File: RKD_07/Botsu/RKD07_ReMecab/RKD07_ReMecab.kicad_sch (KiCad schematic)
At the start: 16 parts, among them J2 Conn_01x24, J3 Qwiic_RA, J4 Conn_01x06, J5 Conn_01x02_Socket, J7 Conn_01x08, J8 Conn_01x06, SW41 SW_Push, U1 Pico

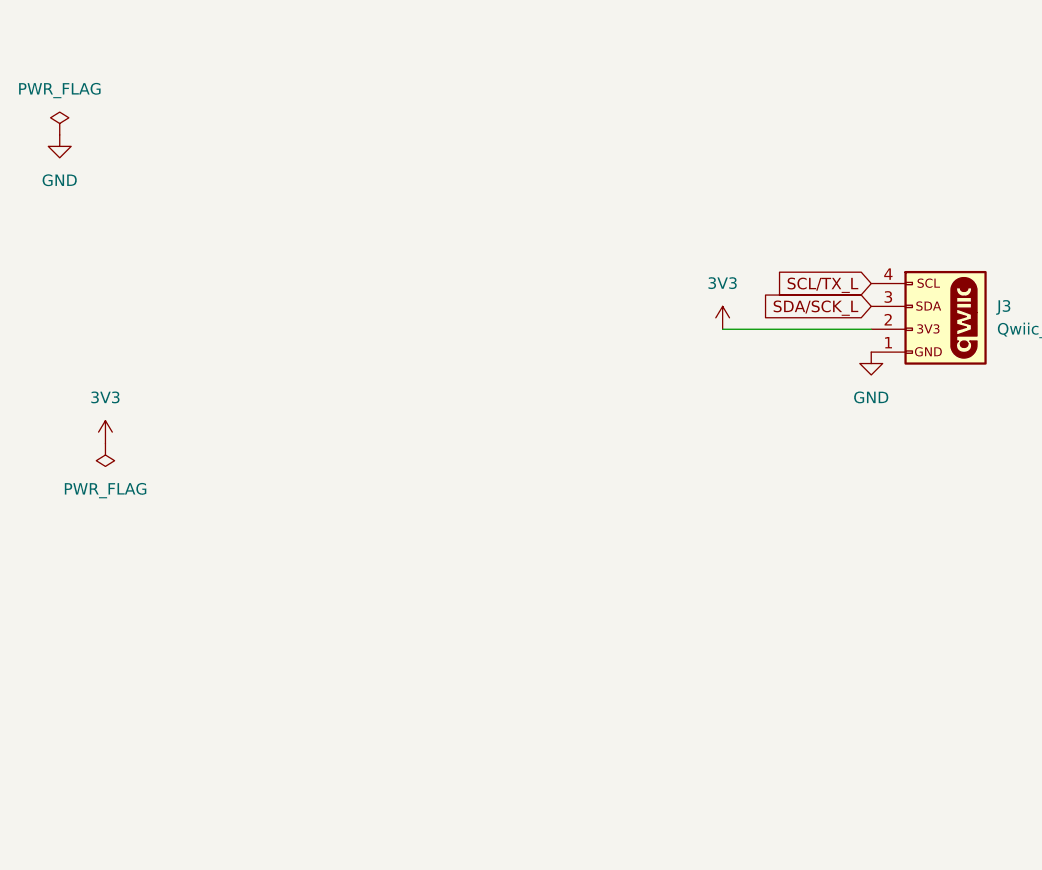
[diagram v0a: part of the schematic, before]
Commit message: Update Remecab
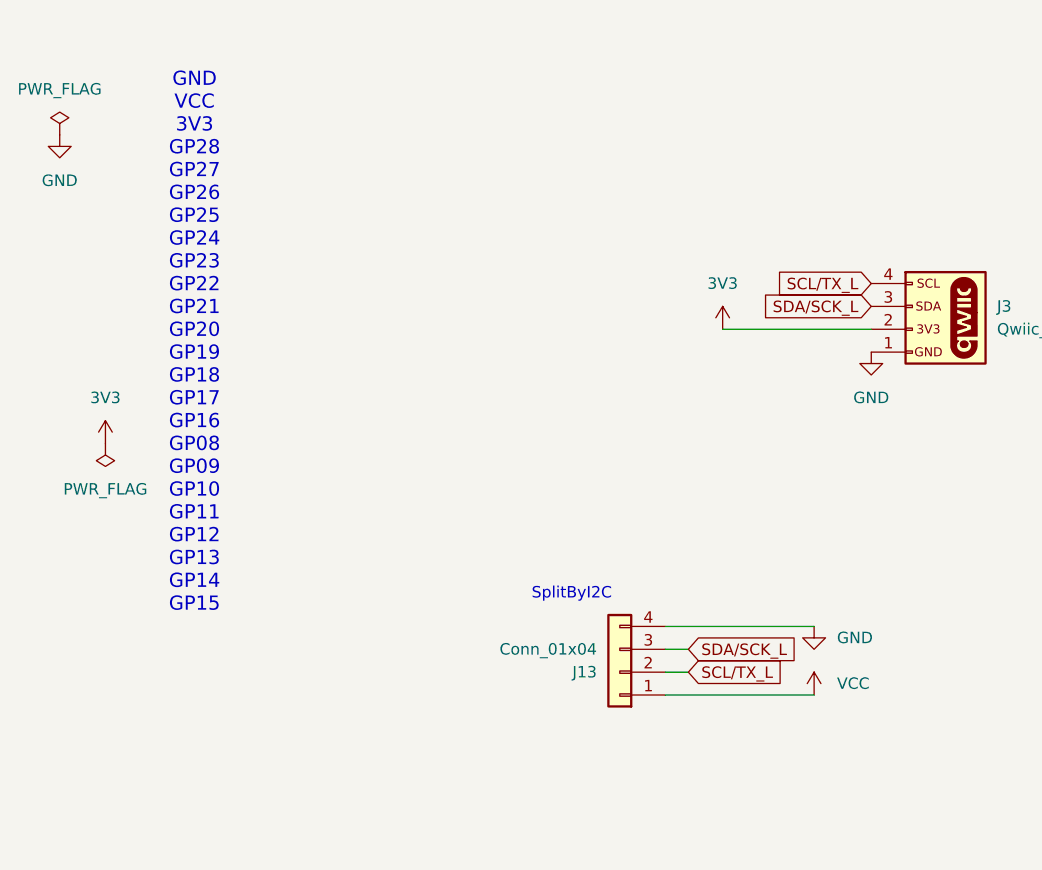
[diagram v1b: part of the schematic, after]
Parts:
- added J13: Conn_01x04, Connector_PinHeader_2.54mm:PinHeader_1x04_P2.54mm_Horizontal, symbol Connector_Generic:Conn_01x04
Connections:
- net GND: now also J13.4 (Pin_4)
- net SCL/TX_L: now also J13.2 (Pin_2)
- net SDA/SCK_L: now also J13.3 (Pin_3)
- net VCC: now also J13.1 (Pin_1)
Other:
- note added: "GND VCC 3V3 GP28 GP27 GP26 GP25 GP24 GP23 GP22 GP21 GP20 GP19 GP18 GP17 GP16 GP08 GP09 GP10 GP11 GP12 GP13 GP14 GP15"
- note added: "SplitByI2C"
